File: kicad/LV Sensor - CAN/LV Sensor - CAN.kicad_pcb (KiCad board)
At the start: 2 copper layers, 29.8 x 29.2 mm, 9 parts, among them J2 Conn_01x09_Pin, U1 MCP2518FD-xJHA, U2 DSC1001DL5-020.0000T, U5 ATA6561-GAQW-N

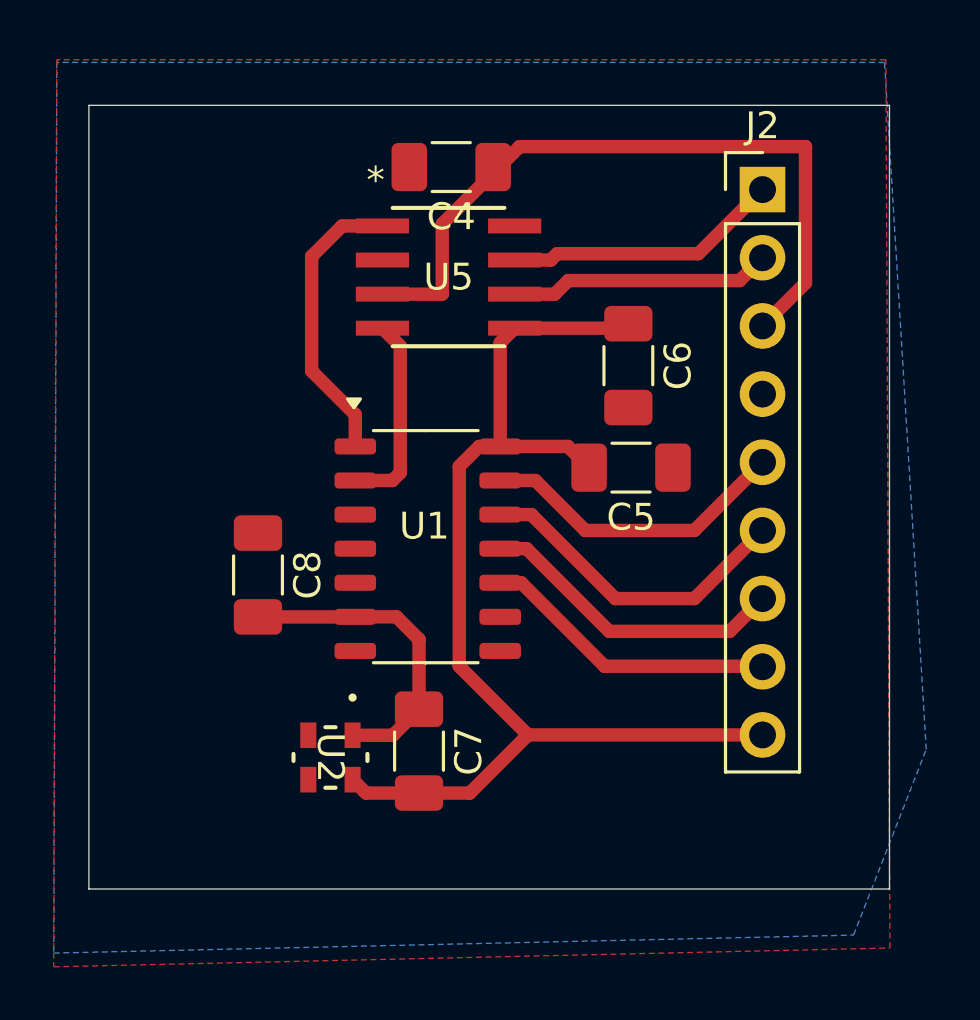
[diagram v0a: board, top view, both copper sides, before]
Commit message: 09-06-2025 Final CAN Board
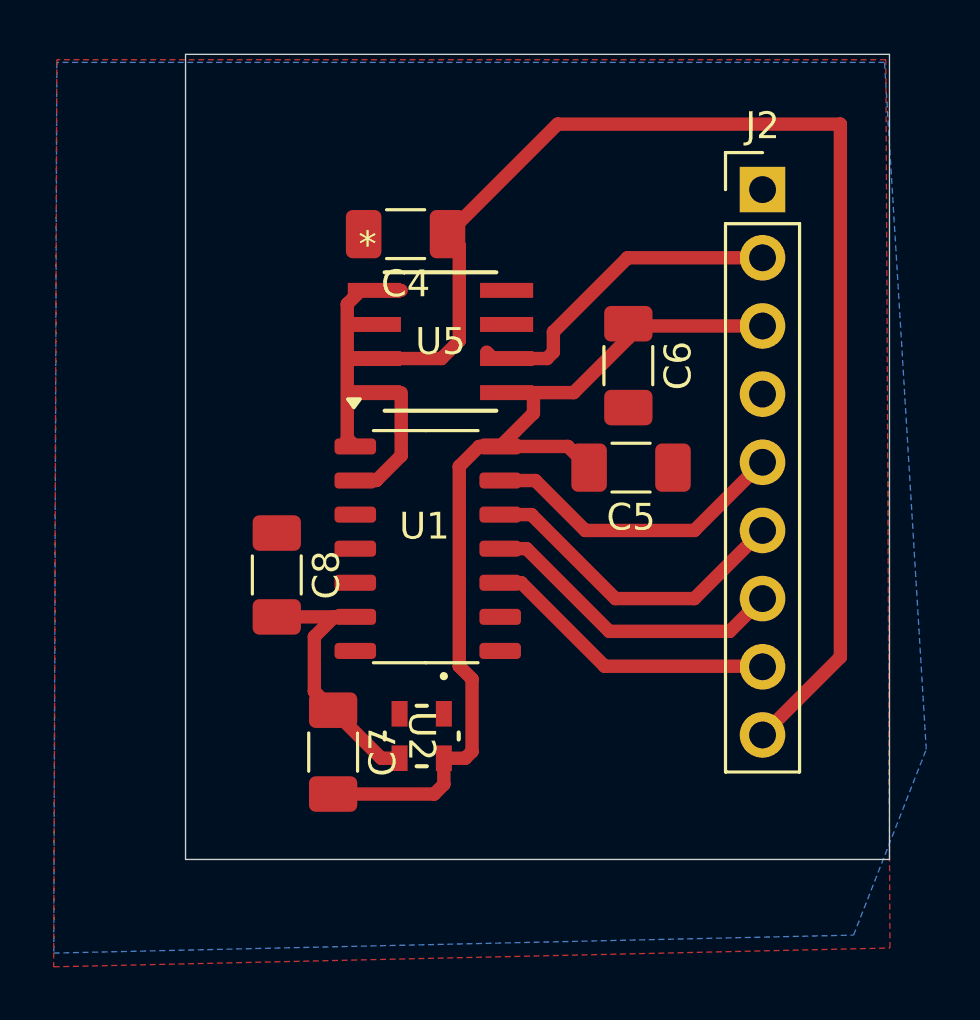
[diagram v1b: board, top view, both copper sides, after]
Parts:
- moved U2 3.49 mm to (114.5, 55.8)
- moved C7 3.20 mm to (111.2, 56.4)
- moved C4 3.02 mm to (113.9, 37.1)
- moved U5 2.42 mm to (115.2, 41.1)
- moved C8 0.70 mm to (109.1, 49.8)
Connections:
- C7 pad 1: /*STANDBY -> Net-(U1-OSC1)
- C8 pad 2: /*STANDBY -> Net-(U1-OSC1)
- J2 pad 3: +5V -> +3.3V
- J2 pad 9: +3.3V -> +5V
- U1 pad 6: /*STANDBY -> Net-(U1-OSC1)
- U2 pad 1: /*STANDBY -> unconnected-(U2-*STANDBY-Pad1)
- U2 pad 3: unconnected-(U2-OUT-Pad3) -> Net-(U1-OSC1)
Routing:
- net +5V: track 26.9 -> 46.9 mm
- net /*STANDBY: track 11.8 -> 0.00 mm
- net Net-(U1-OSC1): track 0.00 -> 11.0 mm
- net /CANH: track 10.3 -> 0.00 mm
- net +3.3V: track 41.9 -> 35.6 mm
- net /CANL: track 9.80 -> 13.4 mm
- net /TXCAN: track 10.9 -> 7.65 mm
- net /RXCAN: track 6.85 -> 4.44 mm
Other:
- board size 29.8 x 29.2 mm -> 26.2 x 30 mm
